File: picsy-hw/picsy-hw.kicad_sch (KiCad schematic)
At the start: 112 parts, among them J1 Power/Data, J2 BATT, J3 Cam, J4 Cam, J5 SD, J6 0.99" Display, J7 2" Display, P2 TC2030-CTX-Tag-Connect, Q1 S8050, Q2 S8050, Q3 AO3401A, SW1 ON/OFF, SW2 RST, SW3 trigger, SW4 trigger, SW5 Rs1010-Resolution-3, SW6 Rs1010-Palette-6, SW7 Rs1010-Brightness-5, U1 CH340C, U2 XC6206-1.2V, U3 TLV62565DBVR, U4 BQ24232HRGTR, U5 XC6206-2.8V, U7 ESP32-WROOM-32D, U8 STM32G030F6Px

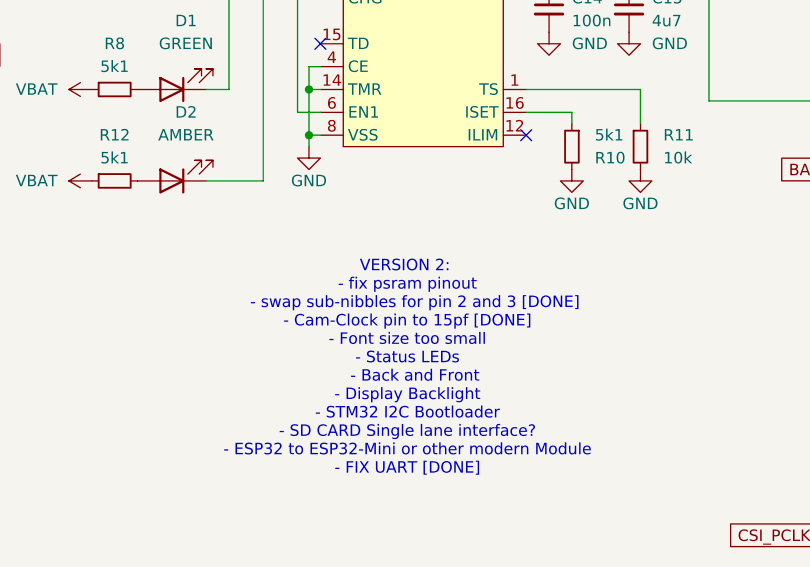
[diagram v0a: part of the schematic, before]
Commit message: updated schematic
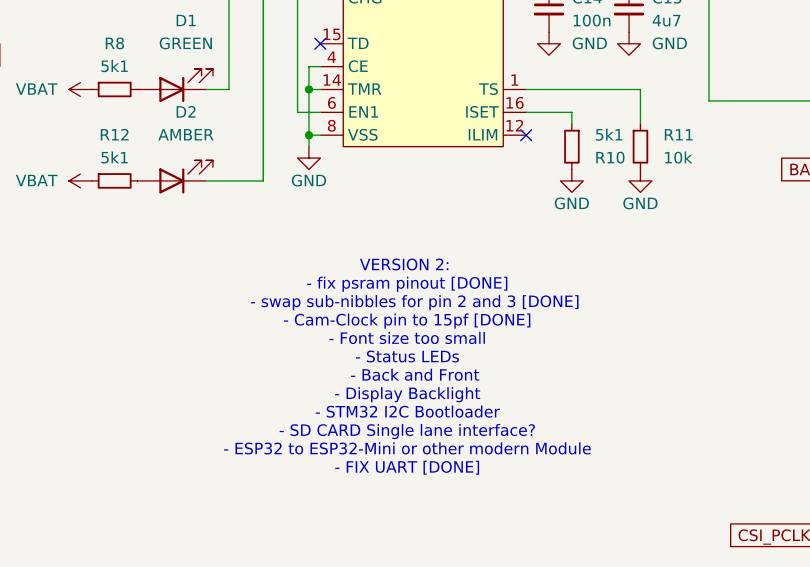
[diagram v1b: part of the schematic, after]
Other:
- note added: "VERSION 2: - fix psram pinout [DONE] - swap sub-nibbles for pin 2 and 3 [DONE] - Cam-Clock pin to 15pf [DONE] - Font size too small - Status LEDs - Back and Front - Display Backlight - STM32 I2C Bootloader - SD CARD Single lane interface? - ESP32 to ESP32-Mini or other modern Module - FIX UART [DONE]"
- note removed: "VERSION 2: - fix psram pinout - swap sub-nibbles for pin 2 and 3 [DONE] - Cam-Clock pin to 15pf [DONE] - Font size too small - Status LEDs - Back and Front - Display Backlight - STM32 I2C Bootloader - SD CARD Single lane interface? - ESP32 to ESP32-Mini or other modern Module - FIX UART [DONE]"
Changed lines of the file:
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@@
 		)
 	)
-	(text "VERSION 2:\n - fix psram pinout\n    - swap sub-nibbles for pin 2 and 3 [DONE]\n - Cam-Clock pin to 15pf [DONE]\n - Font size too small\n - Status LEDs\n	- Back and Front\n - Display Backlight\n - STM32 I2C Bootloader\n - SD CARD Single lane interface?\n - ESP32 to ESP32-Mini or other modern Module\n - FIX UART [DONE]"
+	(text "VERSION 2:\n - fix psram pinout [DONE]\n    - swap sub-nibbles for pin 2 and 3 [DONE]\n - Cam-Clock pin to 15pf [DONE]\n - Font size too small\n - Status LEDs\n	- Back and Front\n - Display Backlight\n - STM32 I2C Bootloader\n - SD CARD Single lane interface?\n - ESP32 to ESP32-Mini or other modern Module\n - FIX UART [DONE]"
 		(exclude_from_sim no)
 		(at 102.108 80.518 0)

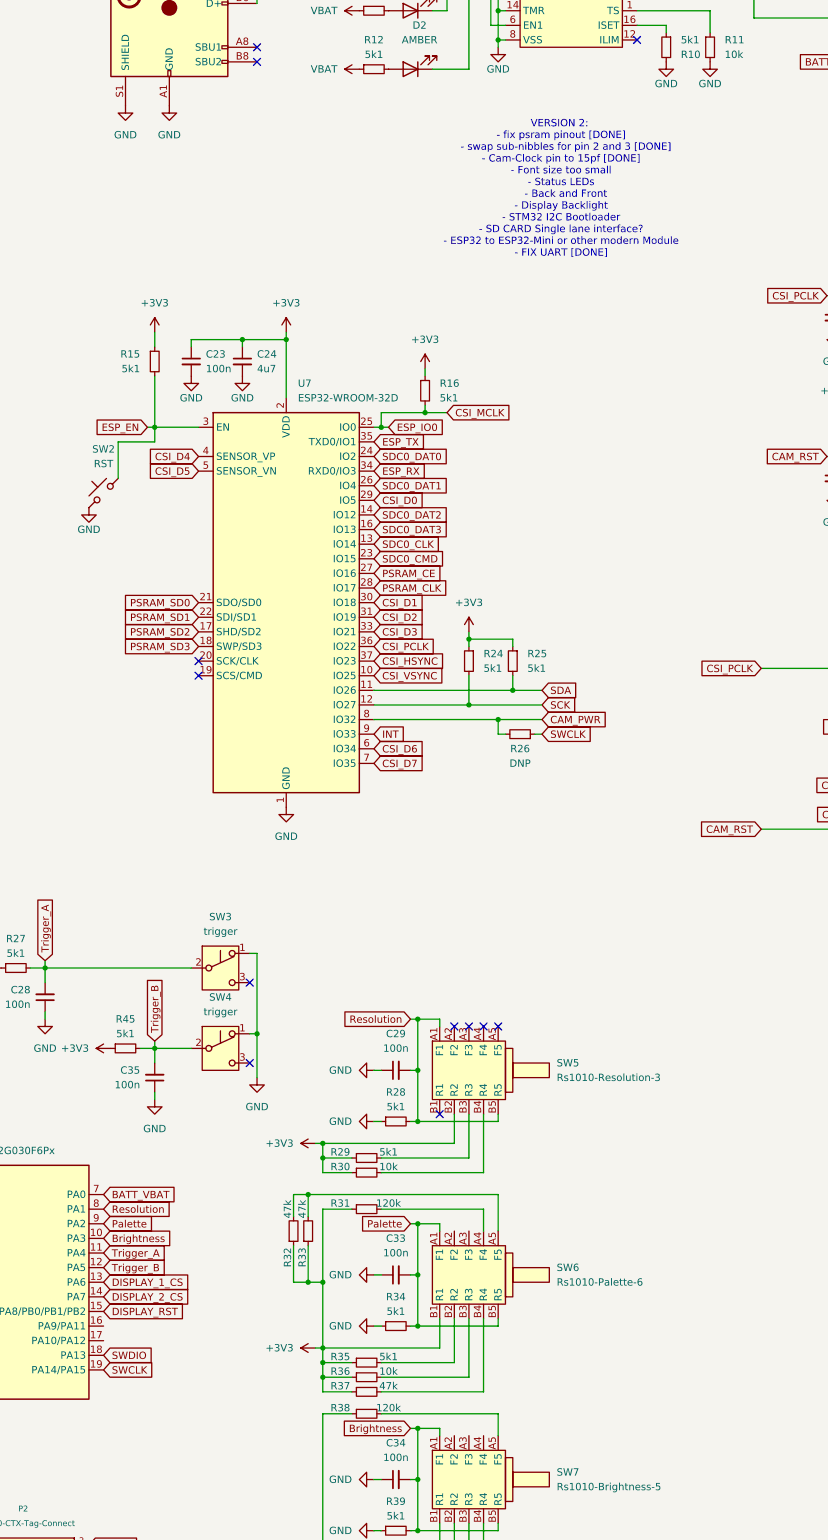
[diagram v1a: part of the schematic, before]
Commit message: updated schematic todo
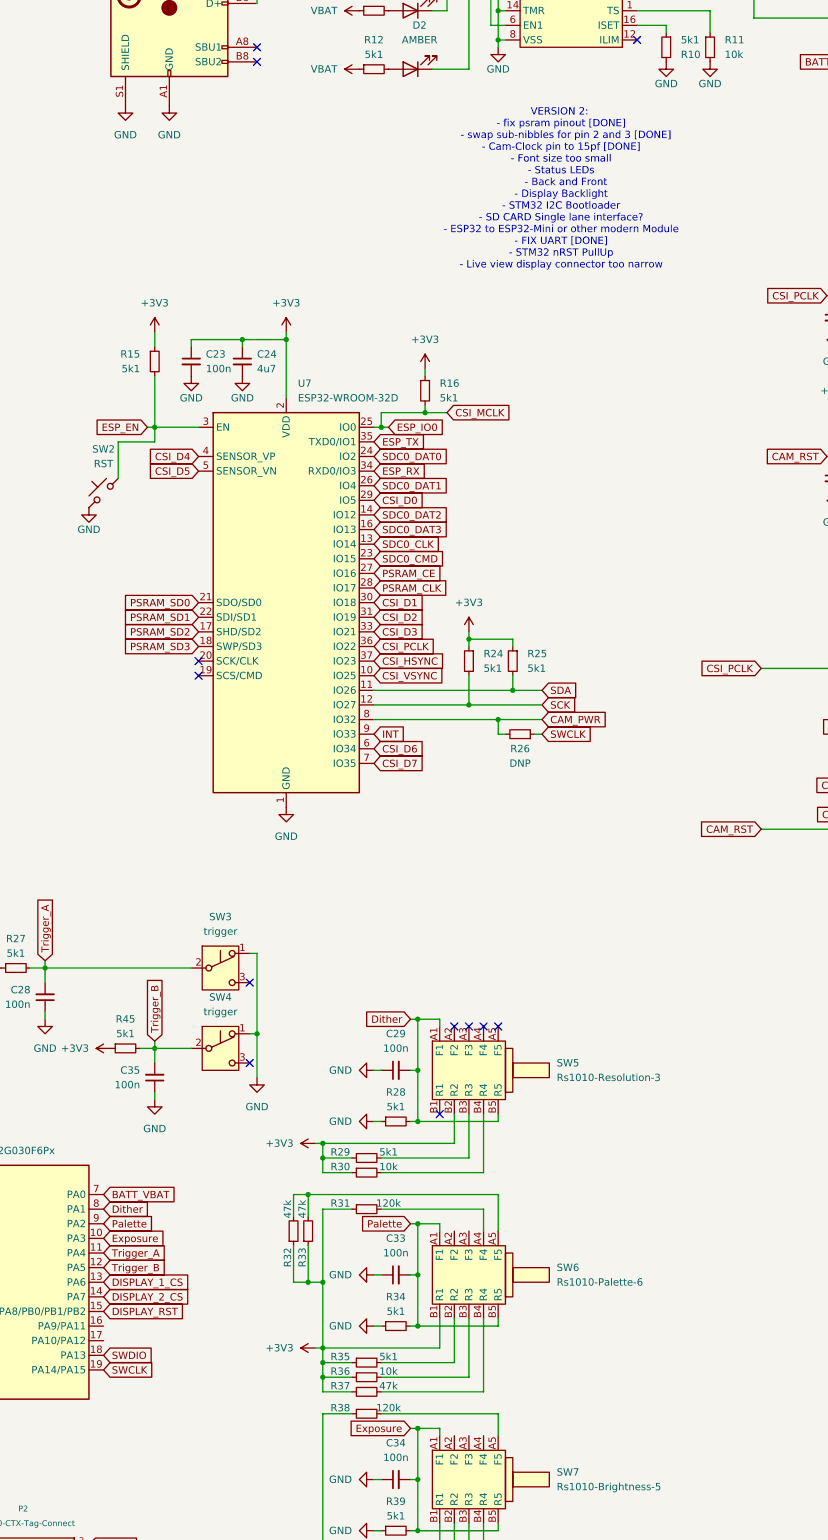
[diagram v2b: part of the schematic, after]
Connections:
- net Brightness renamed Exposure
- net Resolution renamed Dither
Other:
- note added: "VERSION 2: - fix psram pinout [DONE] - swap sub-nibbles for pin 2 and 3 [DONE] - Cam-Clock pin to 15pf [DONE] - Font size too small - Status LEDs - Back and Front - Display Backlight - STM32 I2C Bootloader - SD CARD Single lane interface? - ESP32 to ESP32-Mini or other modern Module - FIX UART [DONE] - STM32 nRST PullUp - Live view display connector too narrow"
- note removed: "VERSION 2: - fix psram pinout [DONE] - swap sub-nibbles for pin 2 and 3 [DONE] - Cam-Clock pin to 15pf [DONE] - Font size too small - Status LEDs - Back and Front - Display Backlight - STM32 I2C Bootloader - SD CARD Single lane interface? - ESP32 to ESP32-Mini or other modern Module - FIX UART [DONE]"
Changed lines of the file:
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@@
 		)
 	)
-	(text "VERSION 2:\n - fix psram pinout [DONE]\n    - swap sub-nibbles for pin 2 and 3 [DONE]\n - Cam-Clock pin to 15pf [DONE]\n - Font size too small\n - Status LEDs\n	- Back and Front\n - Display Backlight\n - STM32 I2C Bootloader\n - SD CARD Single lane interface?\n - ESP32 to ESP32-Mini or other modern Module\n - FIX UART [DONE]"
+	(text "VERSION 2:\n - fix psram pinout [DONE]\n    - swap sub-nibbles for pin 2 and 3 [DONE]\n - Cam-Clock pin to 15pf [DONE]\n - Font size too small\n - Status LEDs\n	- Back and Front\n - Display Backlight\n - STM32 I2C Bootloader\n - SD CARD Single lane interface?\n - ESP32 to ESP32-Mini or other modern Module\n - FIX UART [DONE]\n - STM32 nRST PullUp\n - Live view display connector too narrow"
 		(exclude_from_sim no)
 		(at 102.108 80.518 0)
@@
 		)
 	)
-	(global_label "Brightness"
+	(global_label "Exposure"
 		(shape input)
 		(at 76.2 295.91 180)
@@
 		)
 		(property "Intersheetrefs" "${INTERSHEET_REFS}"
-			(at 63.2363 295.91 0)
+			(at 64.6878 295.91 0)
 			(effects
 				(font
@@
 		)
 	)
-	(global_label "Resolution"
+	(global_label "Dither"
 		(shape input)
 		(at 22.86 257.81 0)
@@
 		)
 		(property "Intersheetrefs" "${INTERSHEET_REFS}"
-			(at 35.8236 257.81 0)
+			(at 31.4695 257.81 0)
 			(effects
 				(font
@@
 		)
 	)
-	(global_label "Resolution"
+	(global_label "Dither"
 		(shape input)
 		(at 76.2 224.79 180)
@@
 		)
 		(property "Intersheetrefs" "${INTERSHEET_REFS}"
-			(at 63.2364 224.79 0)
+			(at 67.5905 224.79 0)
 			(effects
 				(font
@@
 		)
 	)
-	(global_label "Brightness"
+	(global_label "Exposure"
 		(shape input)
 		(at 22.86 262.89 0)
@@
 		)
 		(property "Intersheetrefs" "${INTERSHEET_REFS}"
-			(at 35.8237 262.89 0)
-			(effects
-				(font
+			(at 34.3722 262.89 0)
+			(effects
+				(font
